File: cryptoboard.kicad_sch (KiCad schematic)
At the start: 6 parts, among them J1 USB_A, J2 BOOT, U1 STM32F103C8Tx

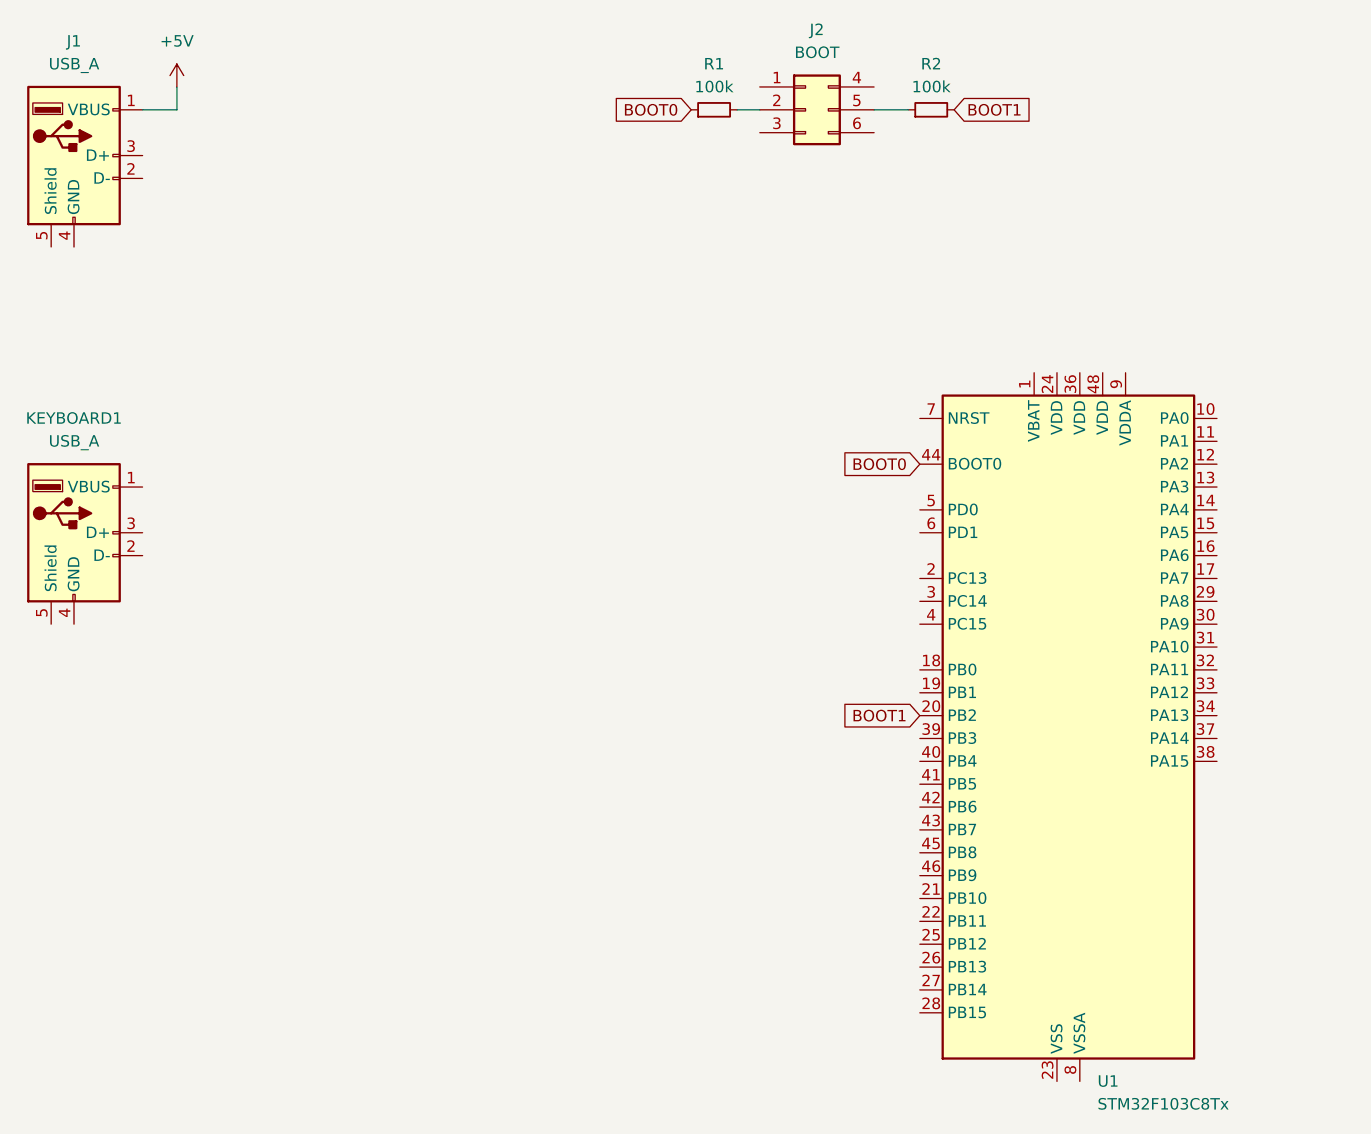
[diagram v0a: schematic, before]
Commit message: add DC DC
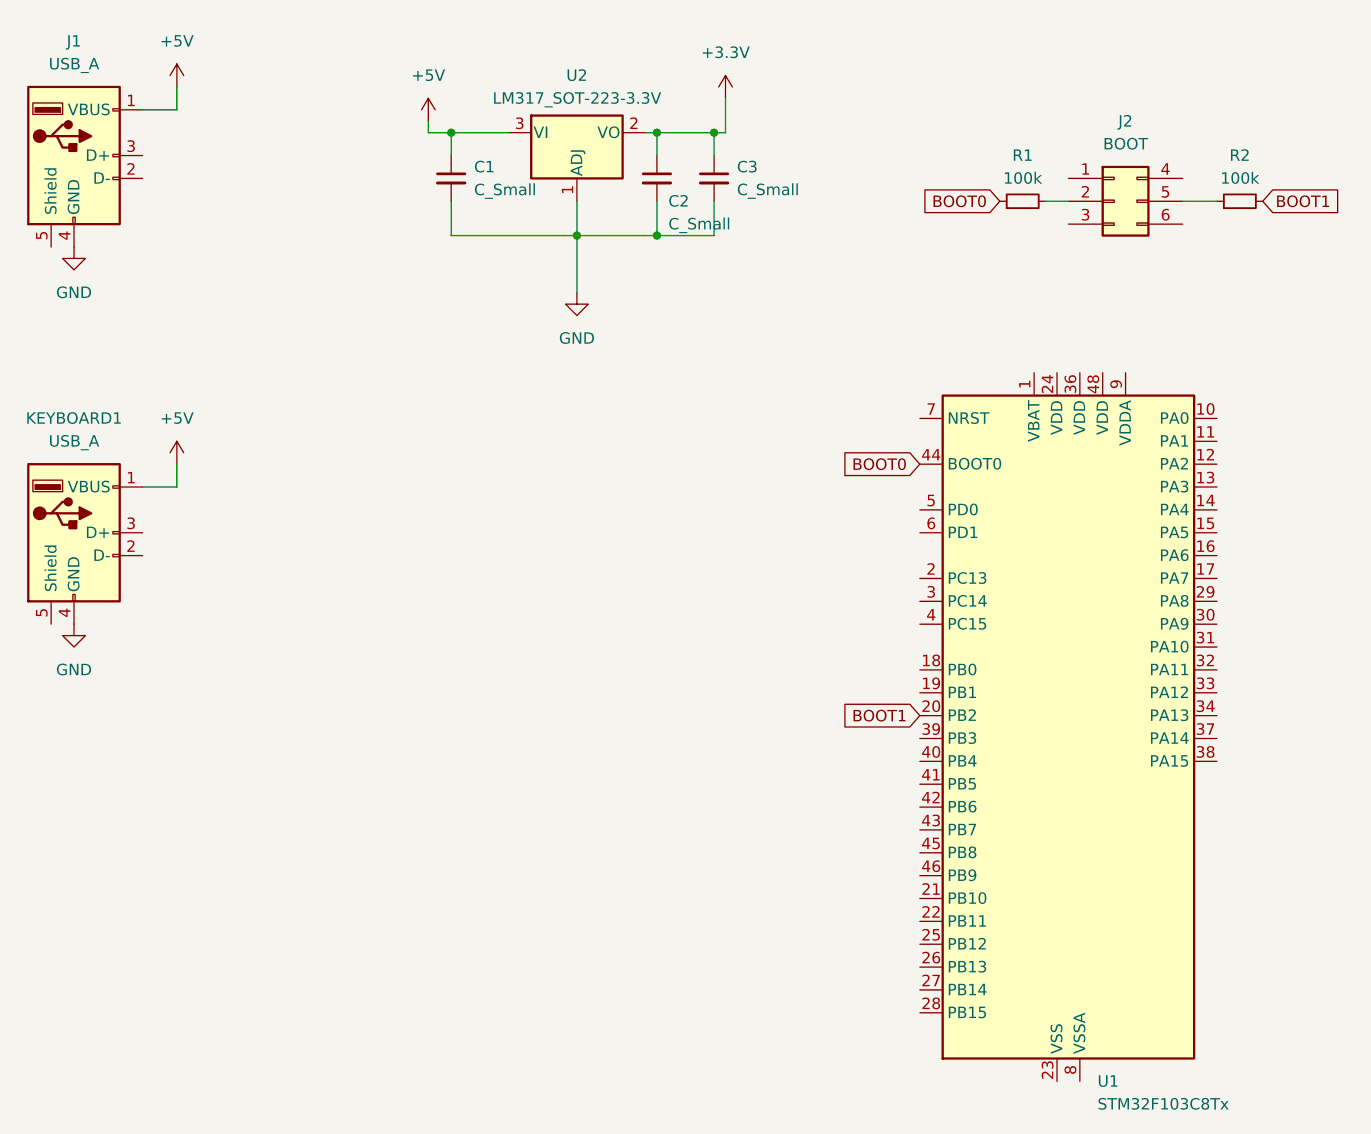
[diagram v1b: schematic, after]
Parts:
- added C1, C2, C3: C_Small, symbol Device:C_Small
- added U2: LM317_SOT-223-3.3V, Package_TO_SOT_SMD:SOT-223-3_TabPin2, symbol Regulator_Linear:LM317_SOT-223
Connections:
- net +5V: now also KEYBOARD1.1 (VBUS), C1.1, U2.3 (VI)
- net GND: now reaches KEYBOARD1.4 (GND)
- net GND: now also J1.4 (GND), C1.2, C2.2, C3.2, U2.1 (ADJ)
- new net +3.3V: C2.1, C3.1, U2.2 (VO)
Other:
- moved on the sheet: J2, R1, R2

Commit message: UPDATE shcema
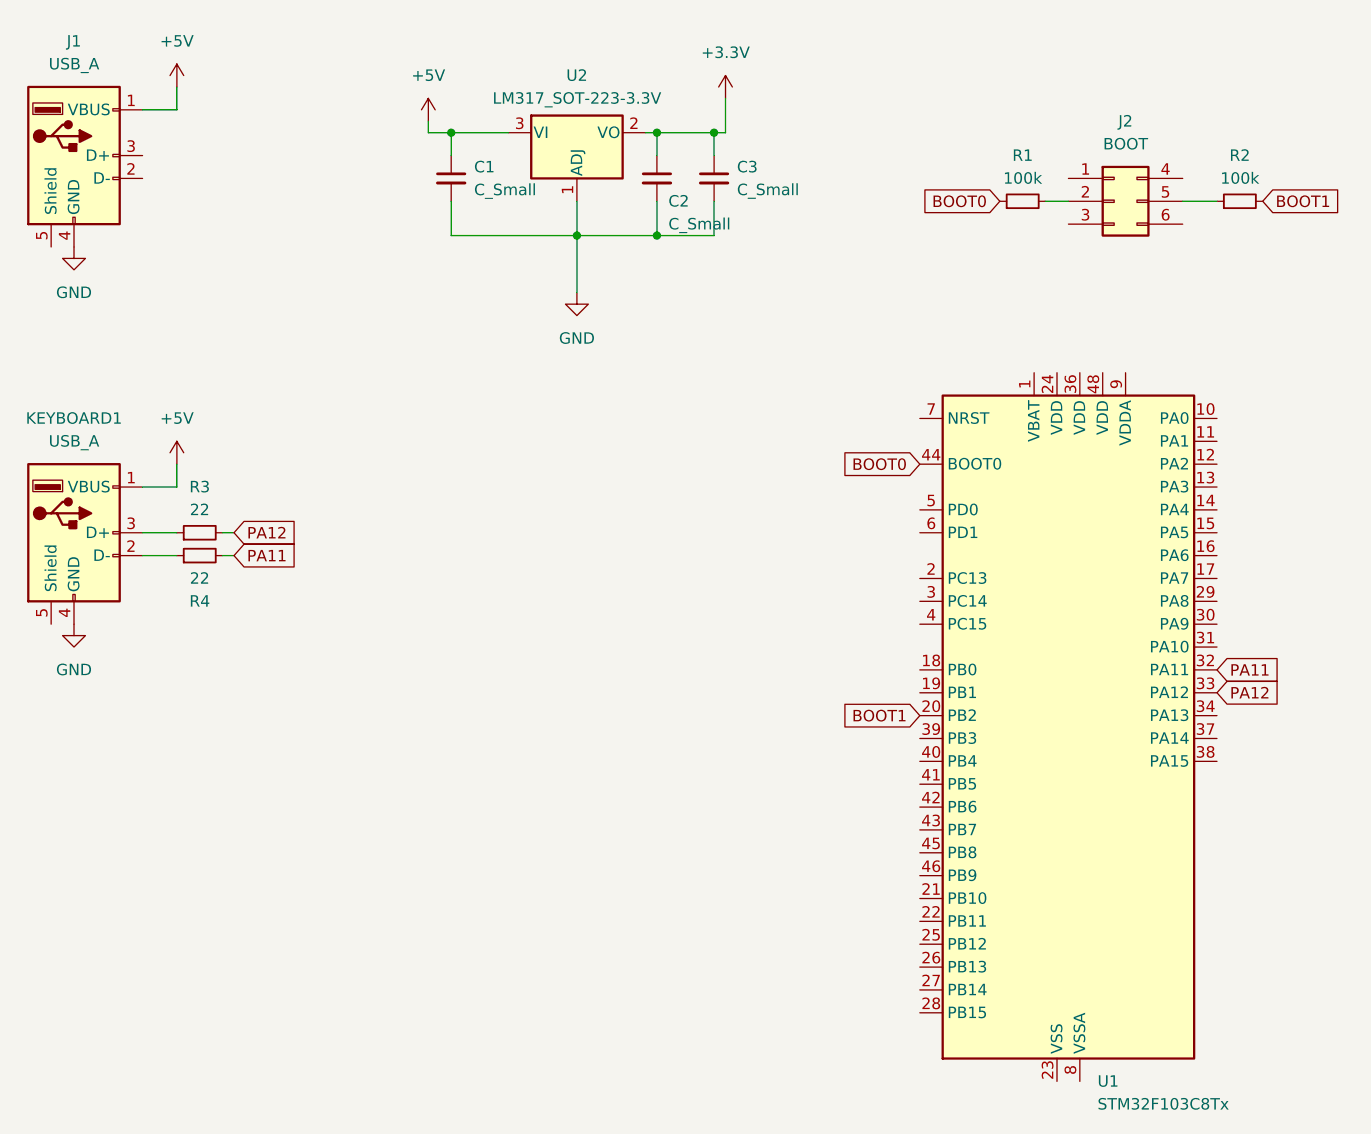
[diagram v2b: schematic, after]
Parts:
- added R3, R4: 22, Resistor_SMD:R_0603_1608Metric, symbol Device:R_Small
- C1, C2, C3: footprint (none) -> Capacitor_SMD:C_0603_1608Metric
- J2: footprint (none) -> Connector_PinHeader_2.54mm:PinHeader_2x03_P2.54mm_Vertical
- R1, R2: footprint (none) -> Resistor_SMD:R_0603_1608Metric
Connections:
- net PA11: now reaches U1.32 (PA11)
- net PA11: now also R4.2
- net PA12: now reaches U1.33 (PA12)
- net PA12: now also R3.2
- net at KEYBOARD1.2 (D-): now also R4.1
- net at KEYBOARD1.3 (D+): now also R3.1
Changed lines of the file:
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@@
+    (stroke (width 0) (type default))
+  )
+  (wire (pts (xy 40.64 72.39) (xy 39.37 72.39))
     (stroke (width 0) (type default))
   )
@@
     (stroke (width 0) (type default))
   )
+  (wire (pts (xy 40.64 69.85) (xy 39.37 69.85))
+    (stroke (width 0) (type default))
+  )
   (wire (pts (xy 71.12 25.4) (xy 64.77 25.4))
     (stroke (width 0) (type default))
@@
     (stroke (width 0) (type default))
   )
+  (wire (pts (xy 30.48 69.85) (xy 34.29 69.85))
+    (stroke (width 0) (type default))
+  )
   (wire (pts (xy 95.25 25.4) (xy 93.98 25.4))
     (stroke (width 0) (type default))
@@
   (wire (pts (xy 34.29 64.77) (xy 34.29 62.23))
     (stroke (width 0) (type default))
+  )
+  (wire (pts (xy 30.48 72.39) (xy 34.29 72.39))
+    (stroke (width 0) (type default))
+  )
+  (global_label "PA12" (shape input) (at 40.64 69.85 0) (fields_autoplaced)
+    (effects (font (size 1.27 1.27)) (justify left))
+    (property "Intersheetrefs" "${INTERSHEET_REFS}" (at 48.3234 69.85 0)
+      (effects (font (size 1.27 1.27)) (justify left) hide)
+    )
   )
   (global_label "BOOT1" (shape input) (at 116.84 90.17 180) (fields_autoplaced)
@@
     )
   )
+  (global_label "PA11" (shape input) (at 149.86 85.09 0) (fields_autoplaced)
+    (effects (font (size 1.27 1.27)) (justify left))
+    (property "Intersheetrefs" "${INTERSHEET_REFS}" (at 157.5434 85.09 0)
+      (effects (font (size 1.27 1.27)) (justify left) hide)
+    )
+  )
   (global_label "BOOT1" (shape input) (at 154.94 33.02 0) (fields_autoplaced)
     (effects (font (size 1.27 1.27)) (justify left))
@@
     (property "Intersheetrefs" "${INTERSHEET_REFS}" (at 116.7161 33.02 0)
       (effects (font (size 1.27 1.27)) (justify right) hide)
+    )
+  )
+  (global_label "PA12" (shape input) (at 149.86 87.63 0) (fields_autoplaced)
+    (effects (font (size 1.27 1.27)) (justify left))
+    (property "Intersheetrefs" "${INTERSHEET_REFS}" (at 157.5434 87.63 0)
+      (effects (font (size 1.27 1.27)) (justify left) hide)
+    )
+  )
+  (global_label "PA11" (shape input) (at 40.64 72.39 0) (fields_autoplaced)
+    (effects (font (size 1.27 1.27)) (justify left))
+    (property "Intersheetrefs" "${INTERSHEET_REFS}" (at 48.3234 72.39 0)
+      (effects (font (size 1.27 1.27)) (justify left) hide)
     )
   )
@@
       (effects (font (size 1.27 1.27)) (justify left))
     )
-    (property "Footprint" "" (at 64.77 30.48 0)
+    (property "Footprint" "Capacitor_SMD:C_0603_1608Metric" (at 64.77 30.48 0)
       (effects (font (size 1.27 1.27)) hide)
     )
@@
       (effects (font (size 1.27 1.27)) (justify left))
     )
-    (property "Footprint" "" (at 93.98 30.48 0)
+    (property "Footprint" "Capacitor_SMD:C_0603_1608Metric" (at 93.98 30.48 0)
       (effects (font (size 1.27 1.27)) hide)
     )
@@
       (effects (font (size 1.27 1.27)))
     )
-    (property "Footprint" "" (at 152.4 33.02 0)
+    (property "Footprint" "Resistor_SMD:R_0603_1608Metric" (at 152.4 33.02 0)
       (effects (font (size 1.27 1.27)) hide)
     )
@@
         (path "/dcd2214c-a8e3-4da9-953a-c4b4305fce7d"
           (reference "#PWR02") (unit 1)
+        )
+      )
+    )
+  )
+  (symbol (lib_id "Device:R_Small") (at 36.83 72.39 90) (unit 1)
+    (in_bom yes) (on_board yes) (dnp no)
+    (property "Reference" "R4" (at 36.83 77.47 90)
+      (effects (font (size 1.27 1.27)))
+    )
+    (property "Value" "22" (at 36.83 74.93 90)
+      (effects (font (size 1.27 1.27)))
+    )
+    (property "Footprint" "Resistor_SMD:R_0603_1608Metric" (at 36.83 72.39 0)
+      (effects (font (size 1.27 1.27)) hide)
+    )
+    (property "Datasheet" "~" (at 36.83 72.39 0)
+      (effects (font (size 1.27 1.27)) hide)
+    )
+    (pin "1")
+    (pin "2")
+    (instances
+      (project "cryptoboard"
+        (path "/dcd2214c-a8e3-4da9-953a-c4b4305fce7d"
+          (reference "R4") (unit 1)
         )
       )
@@
       (effects (font (size 1.27 1.27)) (justify left))
     )
-    (property "Footprint" "" (at 87.63 30.48 0)
+    (property "Footprint" "Capacitor_SMD:C_0603_1608Metric" (at 87.63 30.48 0)
       (effects (font (size 1.27 1.27)) hide)
     )
@@
       (effects (font (size 1.27 1.27)))
     )
-    (property "Footprint" "" (at 138.43 33.02 0)
+    (property "Footprint" "Connector_PinHeader_2.54mm:PinHeader_2x03_P2.54mm_Vertical" (at 138.43 33.02 0)
       (effects (font (size 1.27 1.27)) hide)
     )
@@
     )
   )
+  (symbol (lib_id "Device:R_Small") (at 36.83 69.85 90) (unit 1)
+    (in_bom yes) (on_board yes) (dnp no) (fields_autoplaced)
+    (property "Reference" "R3" (at 36.83 64.77 90)
+      (effects (font (size 1.27 1.27)))
+    )
+    (property "Value" "22" (at 36.83 67.31 90)
+      (effects (font (size 1.27 1.27)))
+    )
+    (property "Footprint" "Resistor_SMD:R_0603_1608Metric" (at 36.83 69.85 0)
+      (effects (font (size 1.27 1.27)) hide)
+    )
+    (property "Datasheet" "~" (at 36.83 69.85 0)
+      (effects (font (size 1.27 1.27)) hide)
+    )
+    (pin "1")
+    (pin "2")
+    (instances
+      (project "cryptoboard"
+        (path "/dcd2214c-a8e3-4da9-953a-c4b4305fce7d"
+          (reference "R3") (unit 1)
+        )
+      )
+    )
+  )
   (symbol (lib_id "Device:R_Small") (at 128.27 33.02 90) (unit 1)
     (in_bom yes) (on_board yes) (dnp no) (fields_autoplaced)
@@
       (effects (font (size 1.27 1.27)))
     )
-    (property "Footprint" "" (at 128.27 33.02 0)
-      (effects (font (size 1.27 1.27)) hide)
-    )
+    (property "Footprint" "Resistor_SMD:R_0603_1608Metric" (at 128.27 33.02 0)
+      (effects (font (size 1.27 1.27)) hide)
+    )
